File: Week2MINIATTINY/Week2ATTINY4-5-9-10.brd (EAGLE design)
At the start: 100 x 80 mm, 19 parts

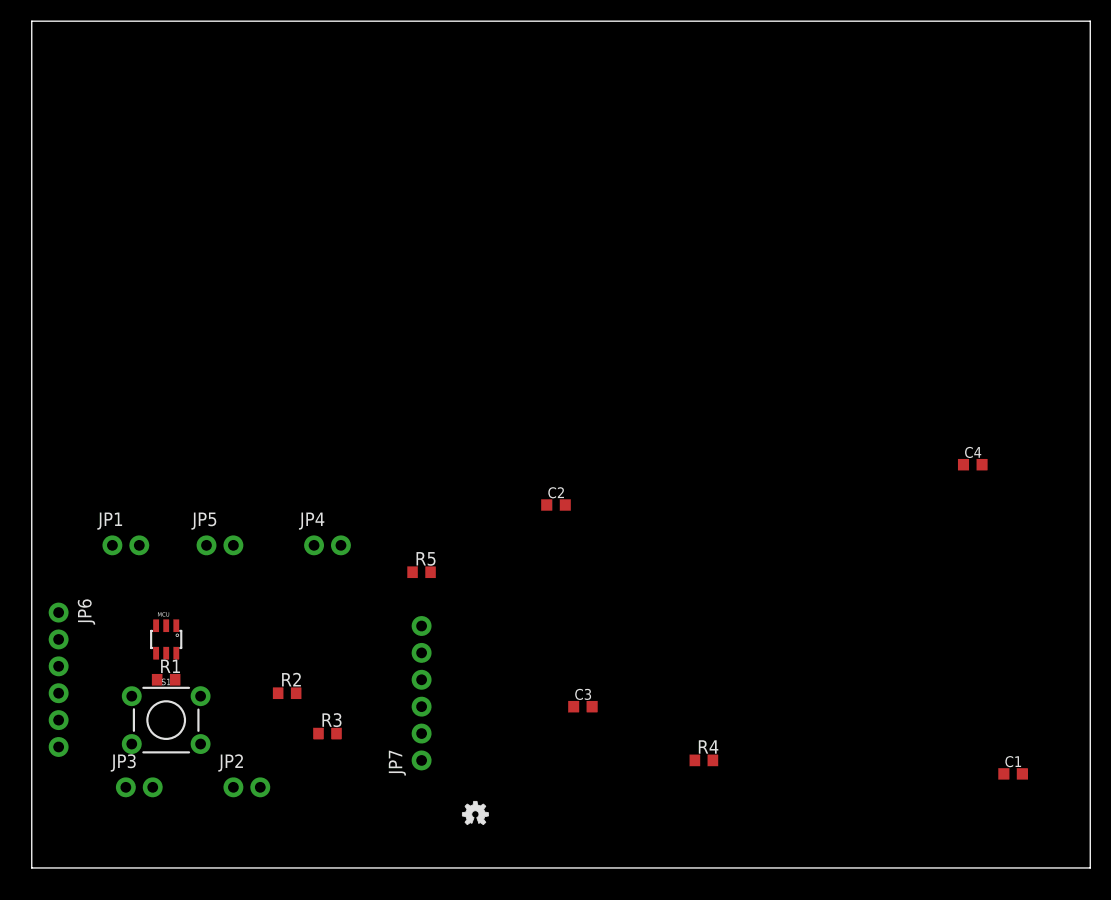
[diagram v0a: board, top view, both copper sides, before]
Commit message: Week2 schmatics finished started Week3
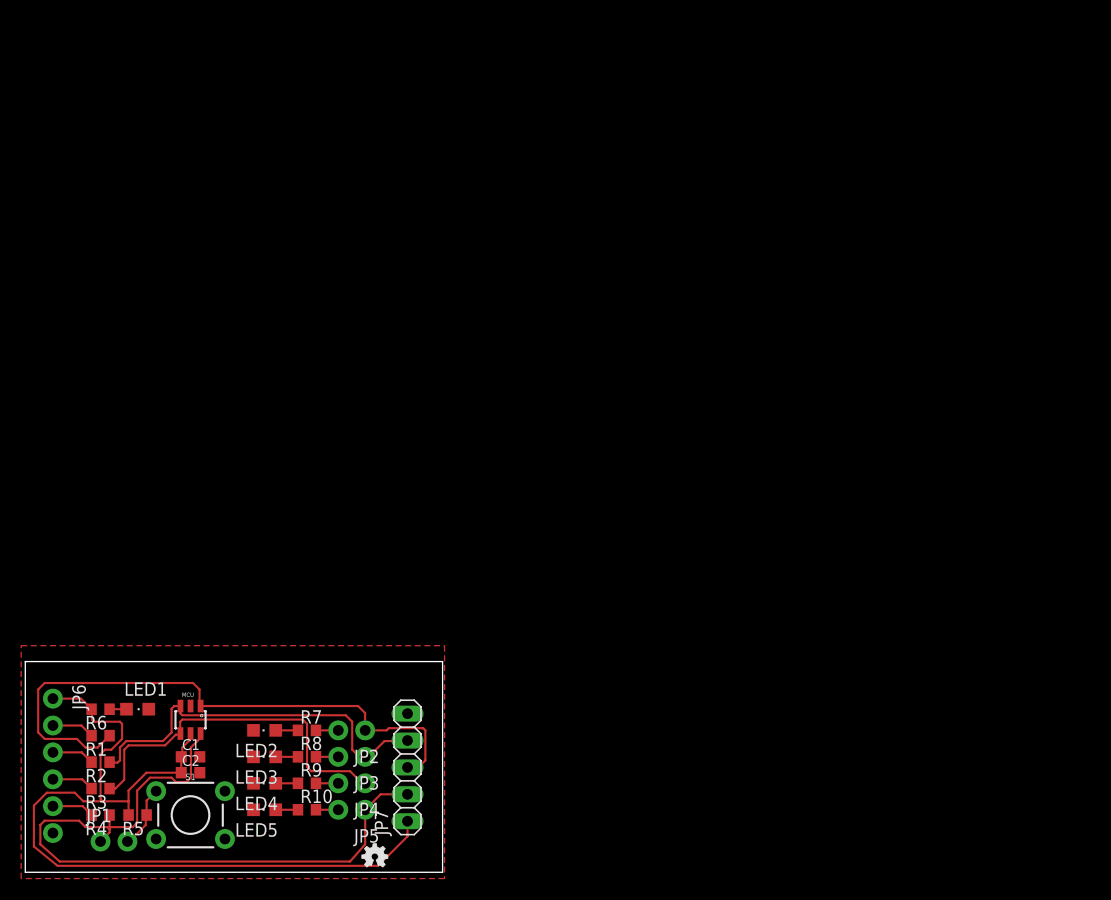
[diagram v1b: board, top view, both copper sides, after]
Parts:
- removed C3, C4: (no value), rcl:C0603K
- added LED1: Power, led:CHIPLED_0805
- added LED2, LED3, LED4, LED5: (no value), led:CHIPLED_0805
- added R10, R6, R7, R8, R9: (no value), rcl:R0603
- JP2: value EXTERNAL_CLK_ENABLE -> LED_SEL_1
- JP3: value M021X02_NO_SILK -> LED_SEL_2
- JP4: value M021X02_NO_SILK -> LED_SEL_3
- JP5: value M021X02_NO_SILK -> LED_SEL_4
- JP7: device SparkFun-Connectors:1X06_NO_SILK -> pinhead:1X05
- moved C1 77.7 mm to (15.0, 10.5)
- moved R4 57.2 mm to (6.50, 5.00), turned to 180 degrees
- moved C2 42.8 mm to (15.0, 9.00)
- moved R5 35.3 mm to (10.0, 5.00), turned to 180 degrees
- moved JP5 29.1 mm to (31.5, 5.50), turned to 180 degrees
- moved JP1 28.0 mm to (6.50, 2.50)
- moved JP4 23.0 mm to (31.5, 8.00), turned to 180 degrees
- moved JP3 22.8 mm to (31.5, 10.5), turned to 180 degrees
- moved R3 22.1 mm to (6.50, 7.50), turned to 180 degrees
- moved R2 18.8 mm to (6.50, 10.0), turned to 180 degrees
- moved JP2 13.6 mm to (31.5, 13.0), turned to 180 degrees
- moved LOGO1 10.3 mm to (32.4, 1.08)
- moved S1 9.26 mm to (15.0, 5.00)
- moved JP6 8.15 mm to (2.00, 16.0)
- moved R1 8.14 mm to (6.50, 12.5), turned to 180 degrees
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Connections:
- new net IOLED1: JP2.2, R7.2
- new net IOLED2: JP3.2, R8.2
- new net IOLED3: JP4.2, R9.2
- new net IOLED4: JP5.2, R10.2
- new net N$1: LED1.A, R6.1
- new net N$2: LED2.A, R7.1
- new net N$3: LED3.A, R8.1
- new net N$4: LED4.A, R9.1
- new net N$5: LED5.A, R10.1
- net GND: now also JP7.5, LED1.C, LED2.C, LED3.C, LED4.C, LED5.C; no longer C3.2, C4.2
- net PB0: now also JP2.1, JP7.3
- net PB1: now also JP3.1, JP7.4
- net PB2: now also JP4.1
- net PB3/_RESET: now also JP5.1, JP7.2
- net VCC: now also JP7.1, R6.2; no longer C3.1, C4.1
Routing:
- net VCC: track 0.00 -> 81.0 mm
- net PB3/_RESET: track 0.00 -> 68.5 mm
- net PB0: track 0.00 -> 57.5 mm
- net PB1: track 0.00 -> 37.0 mm
- net PB2: track 0.00 -> 34.1 mm
- net RESET_PULLUP: track 0.00 -> 5.98 mm
- net IO1: track 0.00 -> 4.05 mm
- net IO2: track 0.00 -> 4.03 mm
- net IO3: track 0.00 -> 4.01 mm
- net IO4: track 0.00 -> 4.00 mm
- net IOLED4: track 0.00 -> 2.11 mm
- net IOLED3: track 0.00 -> 2.11 mm
- net IOLED2: track 0.00 -> 2.11 mm
- net IOLED1: track 0.00 -> 2.11 mm
- net N$5: track 0.00 -> 2.10 mm
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- added copper zone on layer 1, net GND
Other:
- board size 100 x 80 mm -> 39.4 x 19.9 mm
